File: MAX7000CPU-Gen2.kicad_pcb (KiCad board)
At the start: 2 copper layers, 154.9 x 99.3 mm, 128 parts, among them J1 Conn_01x08_Male, J2 Conn_01x08_Male, J3 Conn_01x08_Male, J4 Conn_02x05_Odd_Even, J5 Conn_01x05_Male, SW1 SW_Push, SW2 SW_Push, SW3 SW_Push, U1 NE555P, U10 74LS241, U11 74LS241, U12 AS6C1008-55PCN, U13 74LS574, U14 74LS574, U15 CD4029BEE4, U16 CD4029BEE4, U17 CD4029BEE4, U18 CD4029BEE4, U19 74LS241, U2 NE555P, U20 74LS241, U21 74LS574, U22 74LS574, U23 74LS574, U24 74LS574, U25 74LS574, U26 74LS241, U27 74LS241, U28 EPM7128slc84-15n, U3 NE555P, U4 74LS574, U5 74LS574, U6 CD4029BEE4, U7 CD4029BEE4, U8 CD4029BEE4, U9 CD4029BEE4

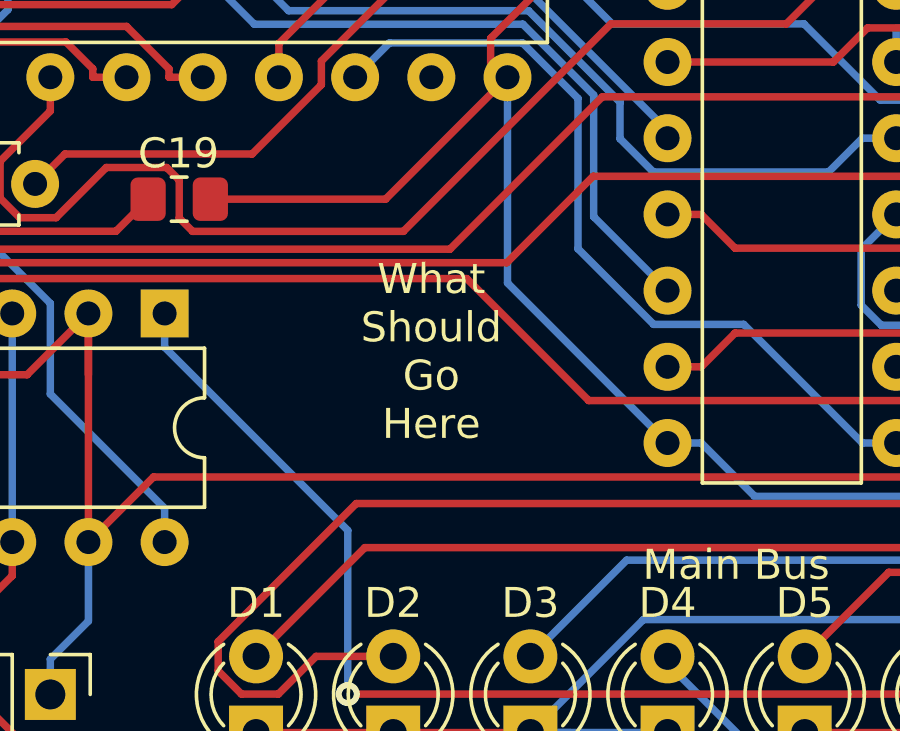
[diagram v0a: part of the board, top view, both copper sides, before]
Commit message: finalized prodcution files
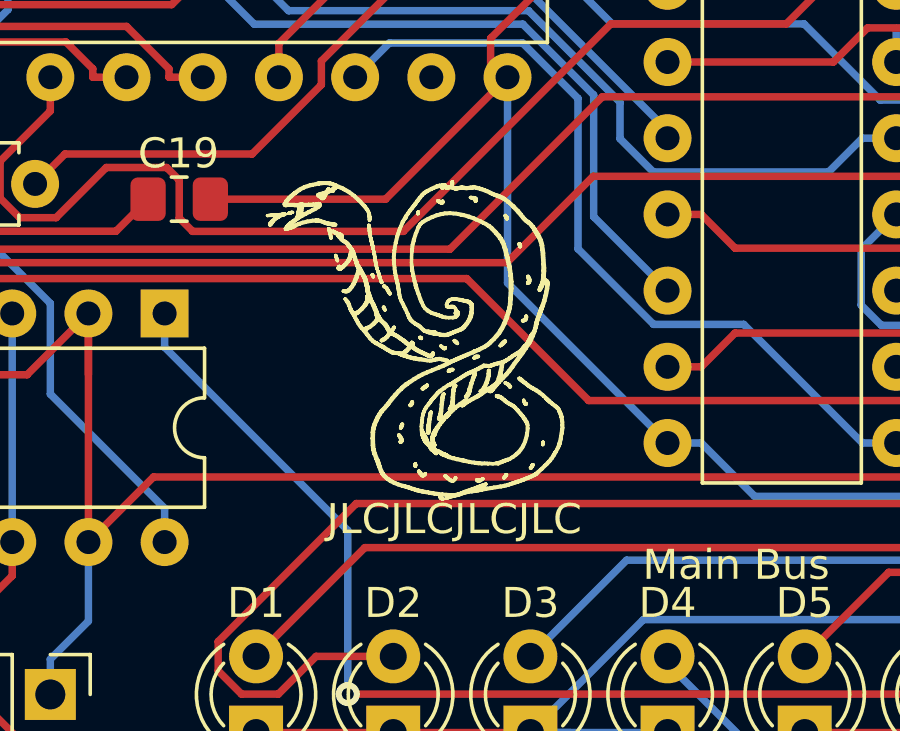
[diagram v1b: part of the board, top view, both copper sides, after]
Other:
- board text added: "JLCJLCJLCJLC"
- board text removed: "What Should Go Here"
